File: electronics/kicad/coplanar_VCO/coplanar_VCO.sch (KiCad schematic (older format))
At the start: 22 parts, among them J1 CONN_01, J2 CONN_01, U1 HMC732, U2 CE3520K3

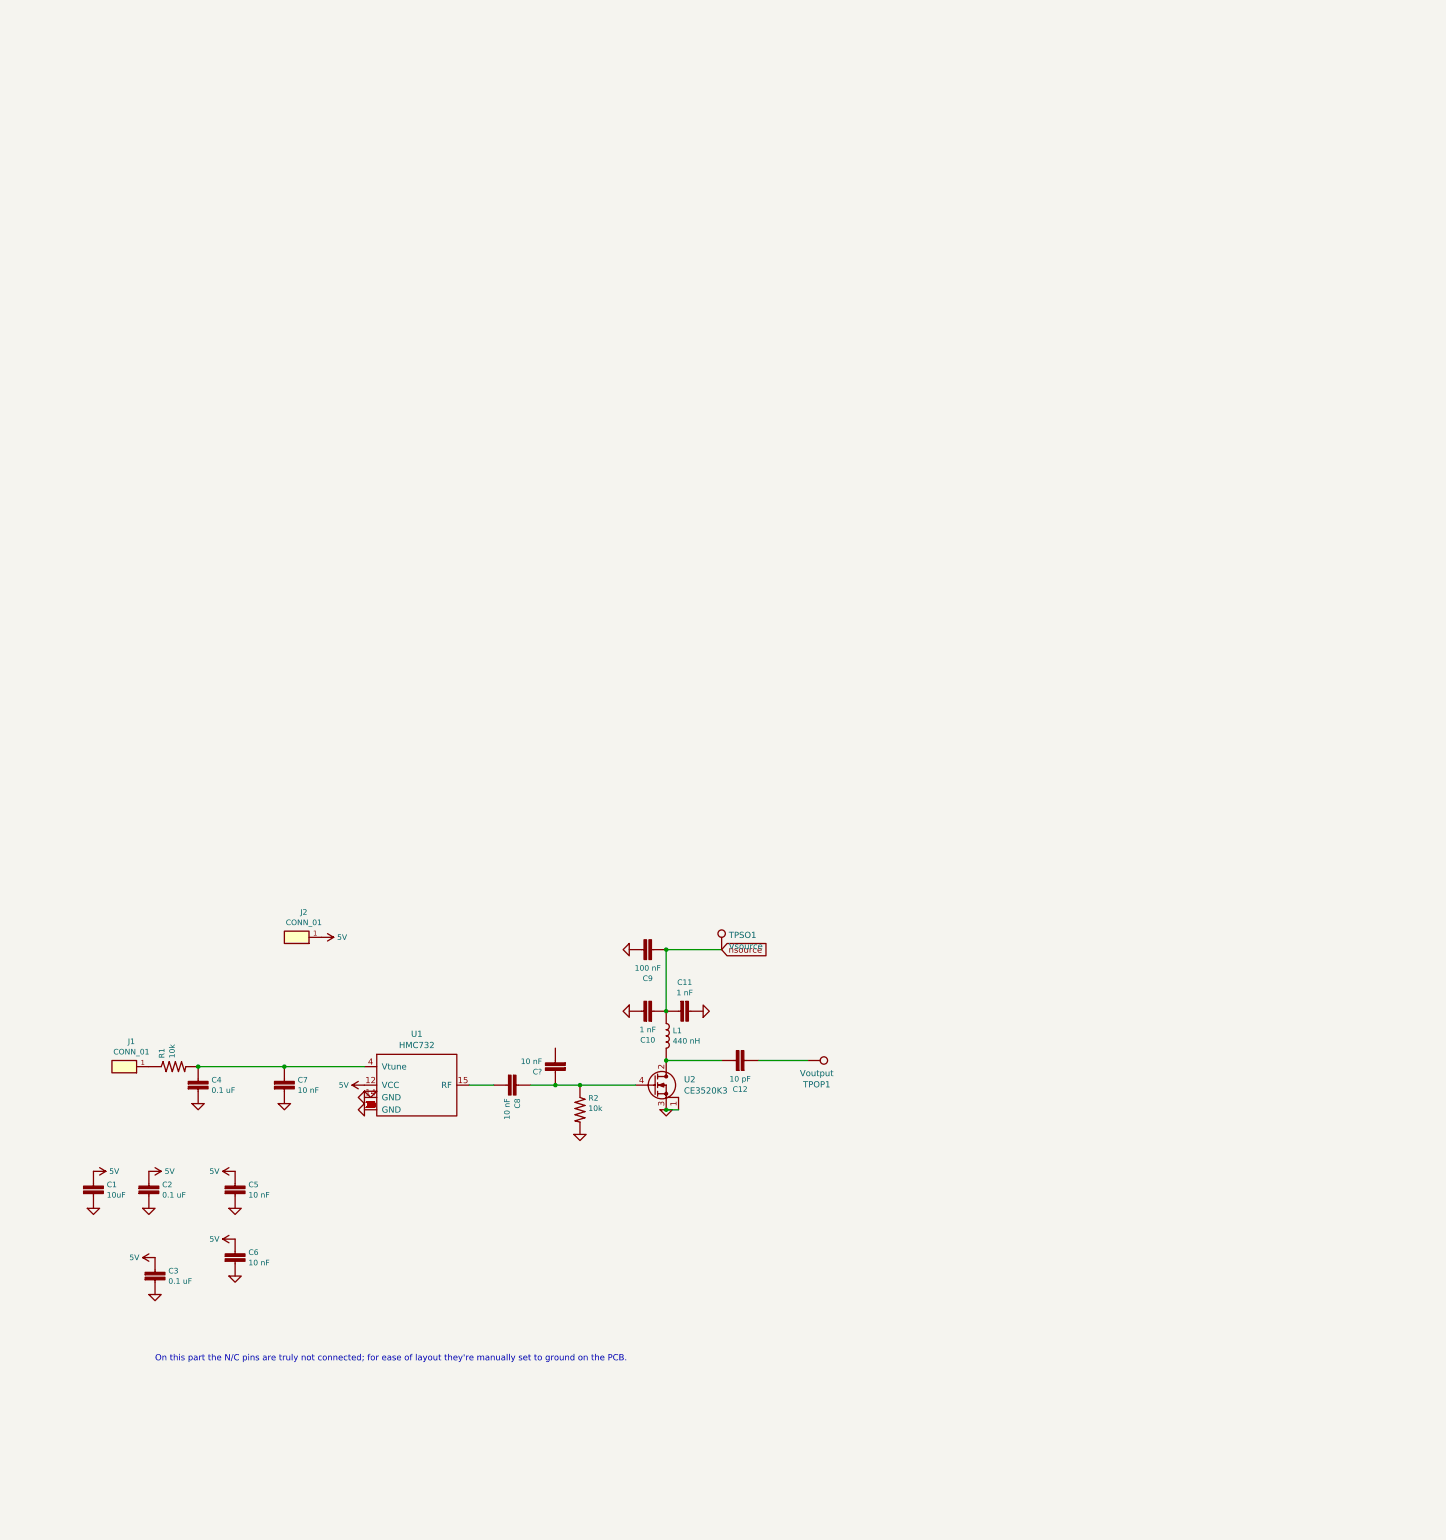
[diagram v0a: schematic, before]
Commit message: Coplanar
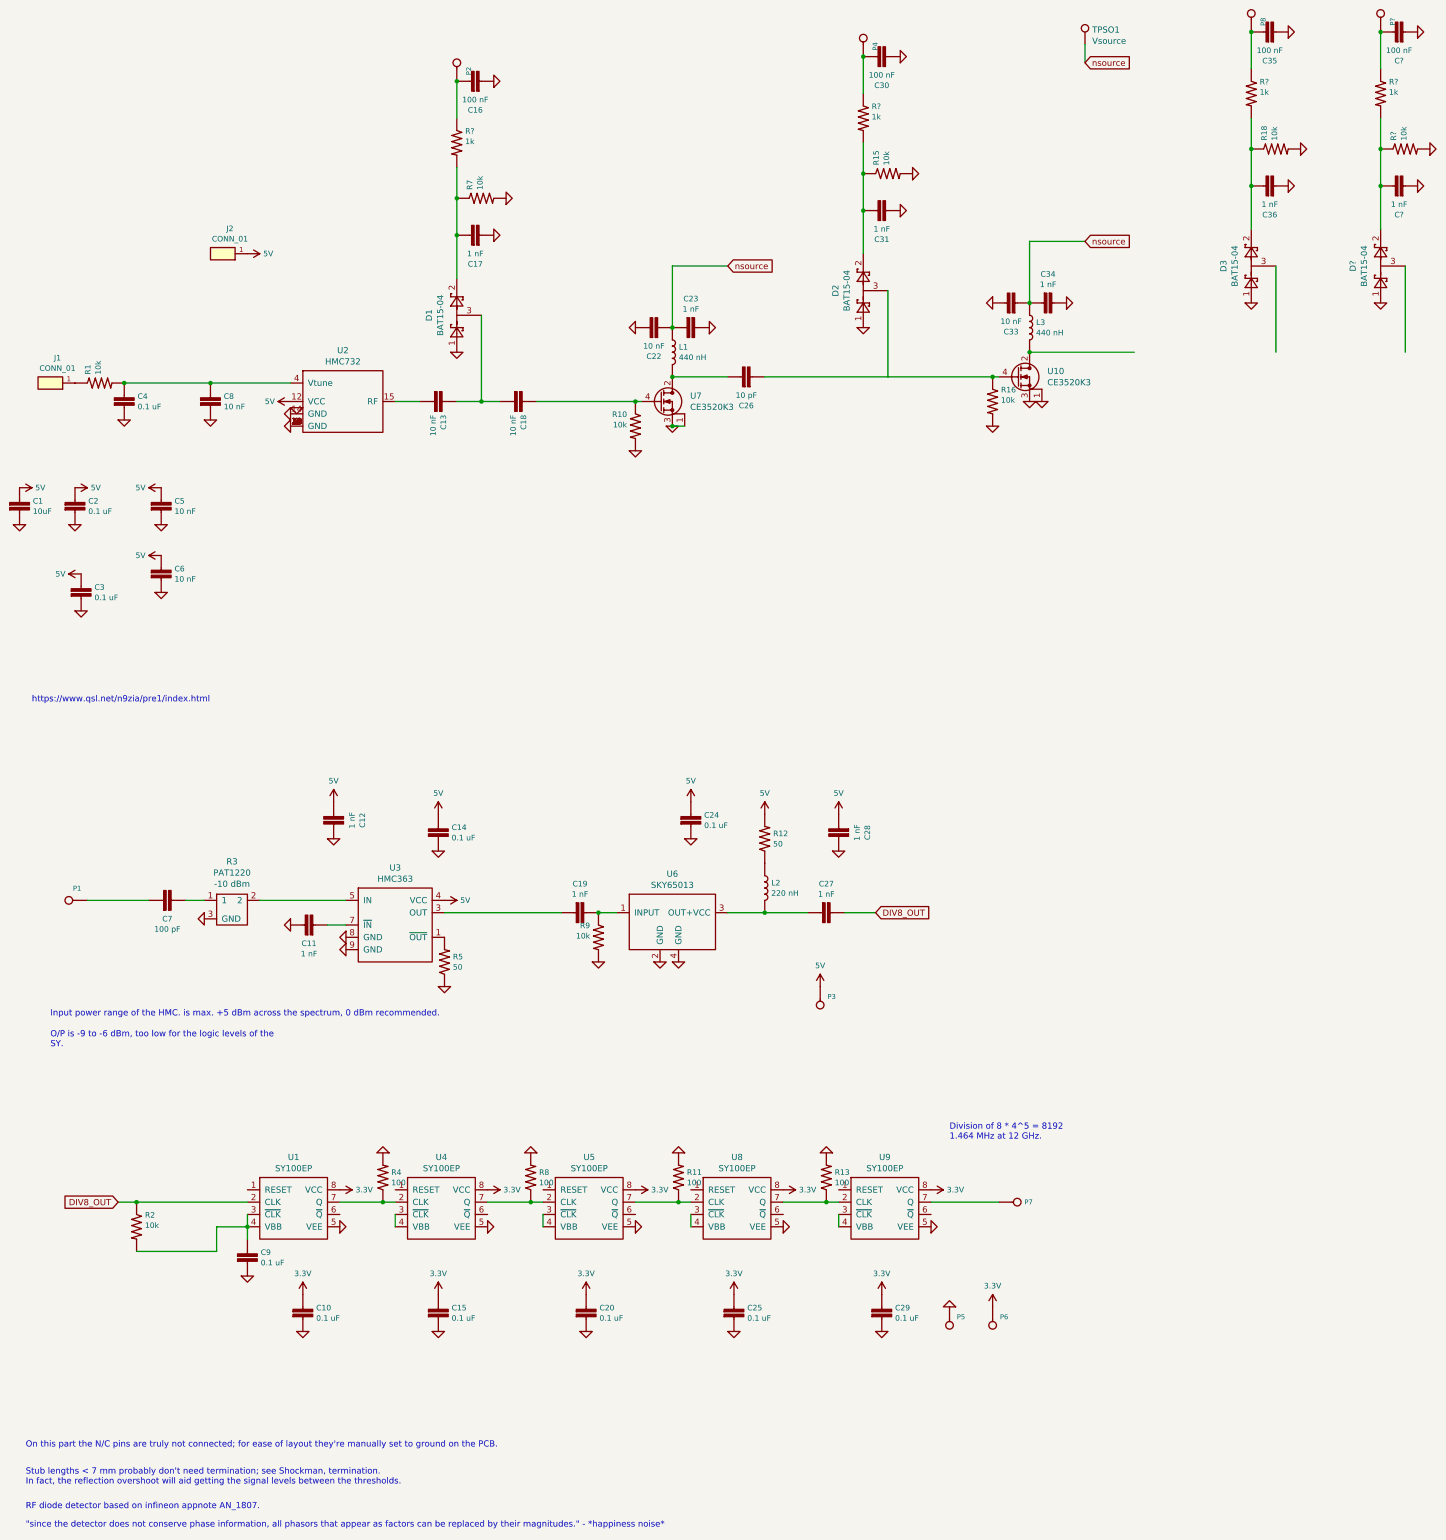
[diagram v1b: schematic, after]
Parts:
- removed C9: 100 nF, 0603, symbol SparkFun-Capacitors:4.7UF0603
- removed C?: 10 nF, 0402, symbol SparkFun-Capacitors:6PF-0402-50V-0.5%
- removed TPOP1: Voutput, TestPoint:TestPoint_Pad_1.0x1.0mm, symbol Connector:Test_Point
- added C10, C14, C15, C20, C24, C25, C29, C9: 0.1 uF, 0603, symbol SparkFun-Capacitors:0.1UF-0603-25V-5%
- added C11, C17, C19, C27, C31, C36, C?: 1 nF, 0402, symbol SparkFun-Capacitors:6PF-0402-50V-0.5%
- added C12, C28, C34: 1 nF, Resistor_SMD:R_0402_1005Metric, symbol SparkFun-Capacitors:4.7UF0603
- added C16, C30, C35, C?: 100 nF, 0603, symbol SparkFun-Capacitors:4.7UF0603
- added C18: 10 nF, 0402, symbol SparkFun-Capacitors:6PF-0402-50V-0.5%
- added C33: 10 nF, Resistor_SMD:R_0402_1005Metric, symbol SparkFun-Capacitors:4.7UF0603
- added C7: 100 pF, 0402, symbol SparkFun-Capacitors:6PF-0402-50V-0.5%
- added D1, D2, D3, D?: BAT15-04, Package_TO_SOT_SMD:SOT-23, symbol Diode:BAS40-04
- added L2: 220 nH, 0402, symbol SparkFun-Coils:INDUCTOR-0402-3.9NH
- added L3: 440 nH, Resistor_SMD:R_0402_1005Metric, symbol SparkFun-Coils:INDUCTOR-0402-3.9NH
- added P1: CONN_1, TestPoint:TestPoint_Pad_1.5x1.5mm, symbol conn:CONN_1
- added P2, P4, P8, P?: a, TestPoint:TestPoint_Pad_1.5x1.5mm, symbol conn:CONN_1
- added P3, P5, P6, P7: OUTPUT, Connector_PinHeader_2.54mm:PinHeader_1x01_P2.54mm_Vertical, symbol conn:CONN_1
- added R11, R13, R4, R8: 100, 0805, symbol SparkFun-Resistors:0.22OHM-0805-1_4W-1%
- added R12, R5: 50, 0805, symbol SparkFun-Resistors:0.22OHM-0805-1_4W-1%
- added R15, R18, R2, R7, R?: 10k, 0402, symbol SparkFun-Resistors:RESISTOR0402
- added R16, R9: 10k, Resistor_SMD:R_0402_1005Metric, symbol SparkFun-Resistors:RESISTOR0402
- added R3: PAT1220, 0xDBFB7:PAT1220, symbol 0xDBFB7:attenuator
- added R? (x4): 1k, Resistor_SMD:R_0603_1608Metric, symbol SparkFun-Resistors:RESISTOR0402
- added U1, U4, U5, U8, U9: SY100EP, Package_SO:SOIC-8_3.9x4.9mm_P1.27mm, symbol 0xDBFB7:SY100EP
- added U10: CE3520K3, 0xDBFB7:4-Micro-X, symbol 0xDBFB7:CE3520K3
- added U3: HMC363, Package_SO:SOIC-8-1EP_3.9x4.9mm_P1.27mm_EP2.35x2.35mm, symbol 0xDBFB7:HMC363
- added U6: SKY65013, Package_TO_SOT_SMD:SOT-89-3_Handsoldering, symbol 0xDBFB7:SKY65013
- C22: renamed from C10; value 1 nF -> 10 nF
- renumbered C8 to C13, C11 to C23, C12 to C26, C7 to C8, R2 to R10, U1 to U2, U2 to U7
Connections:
- net labels added: 3.3V, DIV8_OUT
- wire segments 11 -> 66
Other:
- note added: ""since the detector does not conserve phase information, all phasors that appear as factors can be replaced by their magnitudes." - *happiness noise*"
- note added: "Division of 8 * 4^5 = 8192\n1.464 MHz at 12 GHz."
- note added: "Input power range of the HMC. is max. +5 dBm across the spectrum, 0 dBm recommended.\n"
- note added: "O/P is -9 to -6 dBm, too low for the logic levels of the \nSY."
- note added: "RF diode detector based on infineon appnote AN_1807."
- note added: "Stub lengths < 7 mm probably don't need termination; see Shockman, termination.\nIn fact, the reflection overshoot will aid getting the signal levels between the thresholds."
- note added: "https://www.qsl.net/n9zia/pre1/index.html"
- moved on the sheet: C1, C13, C2, C22, C23, C26, C3, C4, C5, C6, C8, J1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

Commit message: coplanarizing further
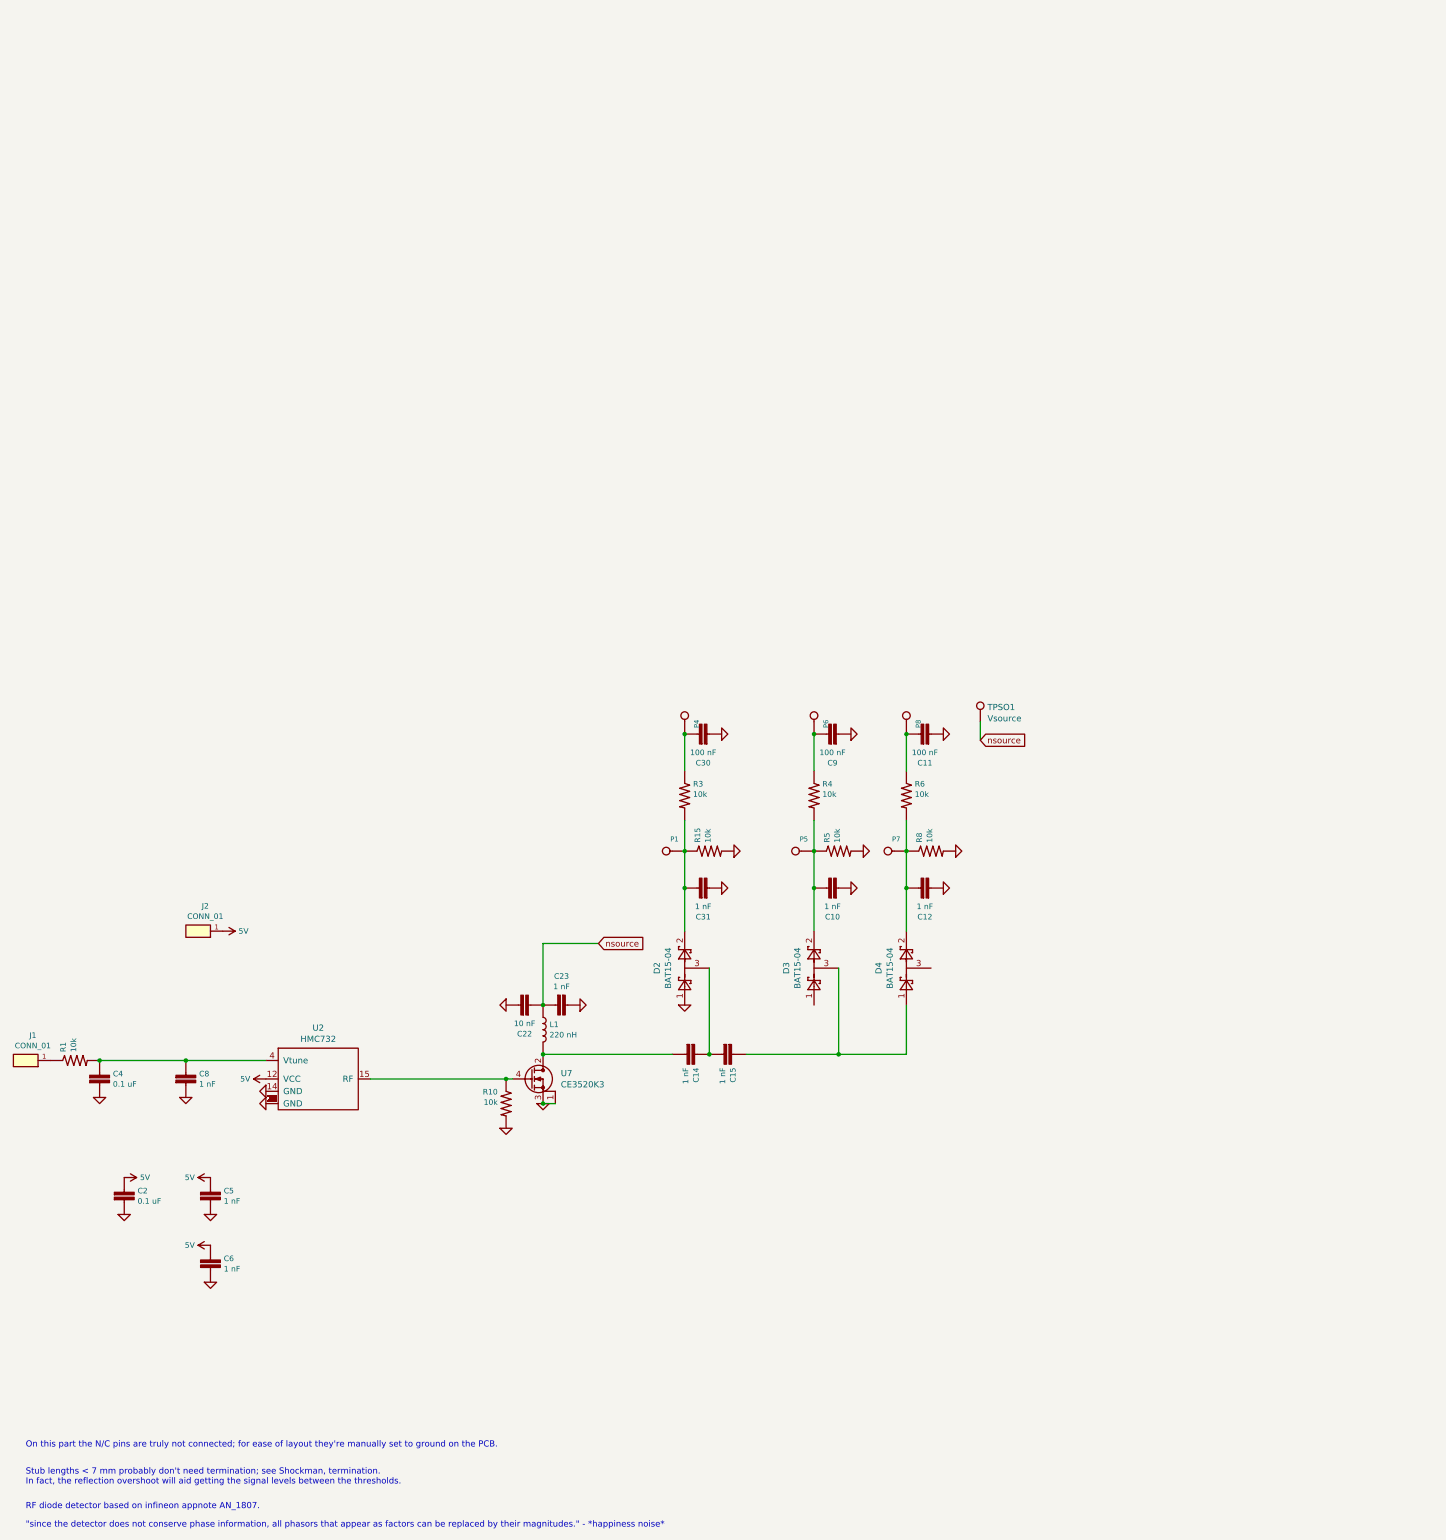
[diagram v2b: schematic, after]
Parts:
- removed C1: 10uF, 1206, symbol SparkFun-Capacitors:1.0UF-1206-50V-10%
- removed C10, C14, C15, C20, C24, C25, C29, C3, C9: 0.1 uF, 0603, symbol SparkFun-Capacitors:0.1UF-0603-25V-5%
- removed C11, C17, C19, C27, C36, C?: 1 nF, 0402, symbol SparkFun-Capacitors:6PF-0402-50V-0.5%
- removed C12, C28, C34: 1 nF, Resistor_SMD:R_0402_1005Metric, symbol SparkFun-Capacitors:4.7UF0603
- removed C13, C18: 10 nF, 0402, symbol SparkFun-Capacitors:6PF-0402-50V-0.5%
- removed C16, C35, C?: 100 nF, 0603, symbol SparkFun-Capacitors:4.7UF0603
- removed C26: 10 pF, Capacitor_SMD:C_0402_1005Metric, symbol SparkFun-Capacitors:6PF-0402-50V-0.5%
- removed C33: 10 nF, Resistor_SMD:R_0402_1005Metric, symbol SparkFun-Capacitors:4.7UF0603
- removed C7: 100 pF, 0402, symbol SparkFun-Capacitors:6PF-0402-50V-0.5%
- removed D1, D?: BAT15-04, Package_TO_SOT_SMD:SOT-23, symbol Diode:BAS40-04
- removed L2: 220 nH, 0402, symbol SparkFun-Coils:INDUCTOR-0402-3.9NH
- removed L3: 440 nH, Resistor_SMD:R_0402_1005Metric, symbol SparkFun-Coils:INDUCTOR-0402-3.9NH
- removed P2, P?: a, TestPoint:TestPoint_Pad_1.5x1.5mm, symbol conn:CONN_1
- removed P3: OUTPUT, Connector_PinHeader_2.54mm:PinHeader_1x01_P2.54mm_Vertical, symbol conn:CONN_1
- removed R11, R13, R4, R8: 100, 0805, symbol SparkFun-Resistors:0.22OHM-0805-1_4W-1%
- removed R12, R5: 50, 0805, symbol SparkFun-Resistors:0.22OHM-0805-1_4W-1%
- removed R16, R9: 10k, Resistor_SMD:R_0402_1005Metric, symbol SparkFun-Resistors:RESISTOR0402
- removed R18, R2, R7, R?: 10k, 0402, symbol SparkFun-Resistors:RESISTOR0402
- removed R3: PAT1220, 0xDBFB7:PAT1220, symbol 0xDBFB7:attenuator
- removed R? (x4): 1k, Resistor_SMD:R_0603_1608Metric, symbol SparkFun-Resistors:RESISTOR0402
- removed U1, U4, U5, U8, U9: SY100EP, Package_SO:SOIC-8_3.9x4.9mm_P1.27mm, symbol 0xDBFB7:SY100EP
- removed U10: CE3520K3, 0xDBFB7:4-Micro-X, symbol 0xDBFB7:CE3520K3
- removed U3: HMC363, Package_SO:SOIC-8-1EP_3.9x4.9mm_P1.27mm_EP2.35x2.35mm, symbol 0xDBFB7:HMC363
- removed U6: SKY65013, Package_TO_SOT_SMD:SOT-89-3_Handsoldering, symbol 0xDBFB7:SKY65013
- added C10, C12, C14, C15: 1 nF, Resistor_SMD:R_0402_1005Metric, symbol SparkFun-Capacitors:6PF-0402-50V-0.5%
- added C11, C9: 100 nF, 0603, symbol SparkFun-Capacitors:4.7UF0603
- added D4: BAT15-04, Package_TO_SOT_SMD:SOT-23, symbol Diode:BAS40-04
- added R3, R4, R5, R6, R8: 10k, Resistor_SMD:R_0402_1005Metric, symbol SparkFun-Resistors:RESISTOR0402
- C31, R15: footprint 0402 -> Resistor_SMD:R_0402_1005Metric
- C5, C6, C8: value 10 nF -> 1 nF
- L1: value 440 nH -> 220 nH
- P1: value CONN_1 -> a
- P5, P6, P7: value OUTPUT -> a; footprint Connector_PinHeader_2.54mm:PinHeader_1x01_P2.54mm_Vertical -> TestPoint:TestPoint_Pad_1.5x1.5mm
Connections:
- net labels removed: 3.3V, DIV8_OUT
- wire segments 66 -> 26
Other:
- note removed: "Division of 8 * 4^5 = 8192\n1.464 MHz at 12 GHz."
- note removed: "Input power range of the HMC. is max. +5 dBm across the spectrum, 0 dBm recommended.\n"
- note removed: "O/P is -9 to -6 dBm, too low for the logic levels of the \nSY."
- note removed: "https://www.qsl.net/n9zia/pre1/index.html"
- moved on the sheet: C2, C22, C23, C30, C31, C4, C5, C6, C8, D2, J1, J2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
